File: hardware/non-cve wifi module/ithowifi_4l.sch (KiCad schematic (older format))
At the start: 48 parts, among them J1 USB_B_Micro, J2 RJ45_LED_Shielded, J3 Conn_Coaxial, J4 Conn_02x02_Odd_Even, J5 Conn_02x02_Odd_Even, J6 Conn_01x02_Male, Q1 BSS138, Q2 BSS138, Q3 BC847, Q4 BC847, SW1 Fail safe, SW2 Reset, U1 ESP32-WROOM, U2 CC1101-868MHz-Module, U3 CH340G, U4 AMS1117-3.3, Y1 Crystal_GND24_Small

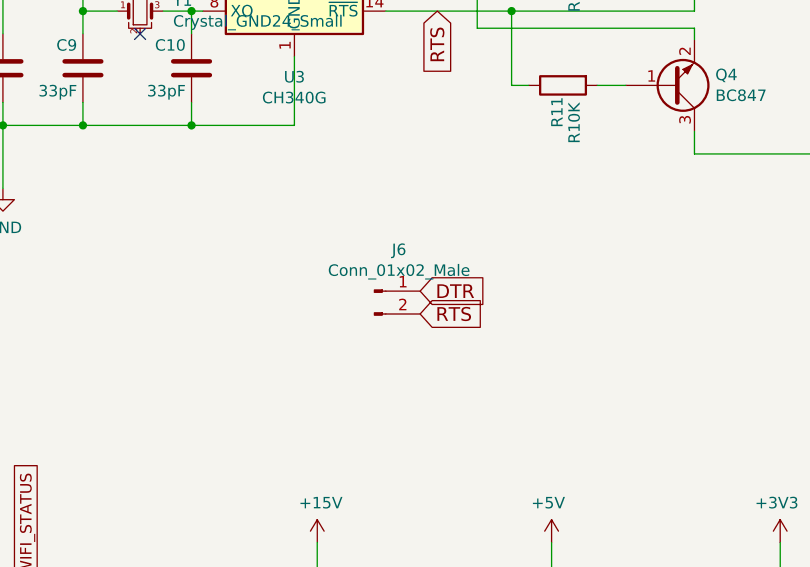
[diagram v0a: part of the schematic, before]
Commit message: Update HW files and correct spelling
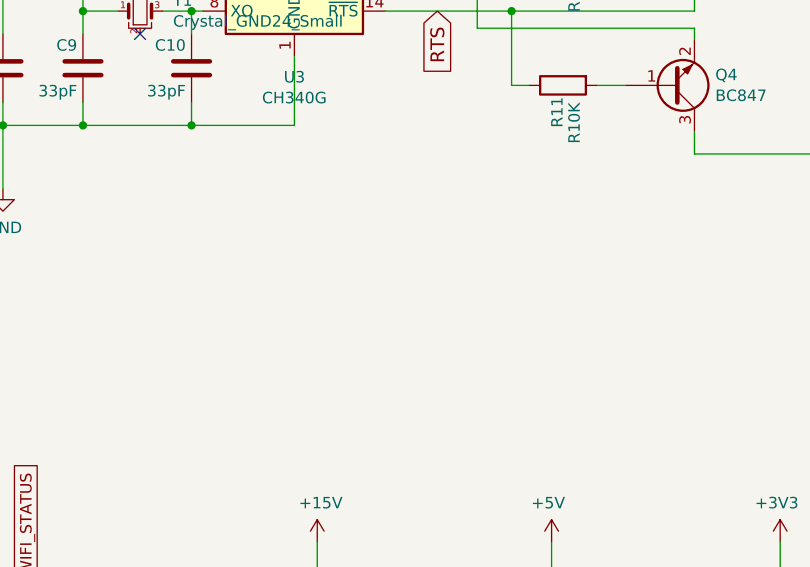
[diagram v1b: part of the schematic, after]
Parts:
- removed J6: Conn_01x02_Male, Connector_PinHeader_2.54mm:PinHeader_1x02_P2.54mm_Vertical, symbol Connector:Conn_01x02_Male
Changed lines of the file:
@@
 Wire Wire Line
 	14525 2450 14600 2450
-$Comp
-L Connector:Conn_01x02_Male J6
-U 1 1 61A92742
-P 3375 4475
-F 0 "J6" H 3483 4656 50  0000 C CNN
-F 1 "Conn_01x02_Male" H 3483 4565 50  0000 C CNN
-F 2 "Connector_PinHeader_2.54mm:PinHeader_1x02_P2.54mm_Vertical" H 3375 4475 50  0001 C CNN
-F 3 "~" H 3375 4475 50  0001 C CNN
-	1    3375 4475
-	1    0    0    -1
-$EndComp
 Wire Wire Line
 	3425 3250 3975 3250
@@
 Text GLabel 3650 3250 3    60   Input ~ 0
 RTS
-Text GLabel 3575 4575 2    60   Input ~ 0
-RTS
-Text GLabel 3575 4475 2    60   Input ~ 0
-DTR
 NoConn ~ 1250 2950
 NoConn ~ 2925 6100

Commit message: Update hardware design files
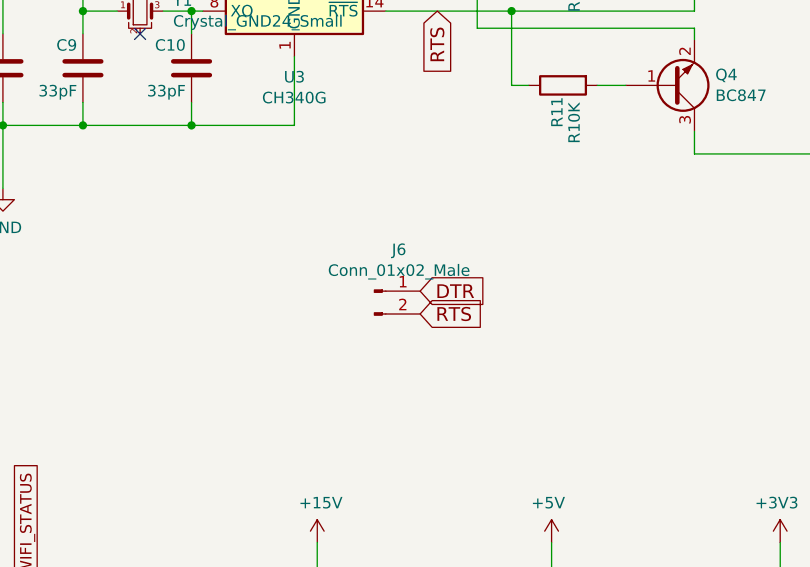
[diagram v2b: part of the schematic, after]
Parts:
- added J6: Conn_01x02_Male, Connector_PinHeader_2.54mm:PinHeader_1x02_P2.54mm_Vertical, symbol Connector:Conn_01x02_Male
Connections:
- net DTR: now also J6.1 (Pin_1)
- net RTS: now also J6.2 (Pin_2)
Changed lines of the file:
@@
 Wire Wire Line
 	14525 2450 14600 2450
+$Comp
+L Connector:Conn_01x02_Male J6
+U 1 1 61A92742
+P 3375 4475
+F 0 "J6" H 3483 4656 50  0000 C CNN
+F 1 "Conn_01x02_Male" H 3483 4565 50  0000 C CNN
+F 2 "Connector_PinHeader_2.54mm:PinHeader_1x02_P2.54mm_Vertical" H 3375 4475 50  0001 C CNN
+F 3 "~" H 3375 4475 50  0001 C CNN
+	1    3375 4475
+	1    0    0    -1
+$EndComp
 Wire Wire Line
 	3425 3250 3975 3250
@@
 Text GLabel 3650 3250 3    60   Input ~ 0
 RTS
+Text GLabel 3575 4575 2    60   Input ~ 0
+RTS
+Text GLabel 3575 4475 2    60   Input ~ 0
+DTR
 NoConn ~ 1250 2950
 NoConn ~ 2925 6100
